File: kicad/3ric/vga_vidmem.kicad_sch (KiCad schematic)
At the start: 9 parts

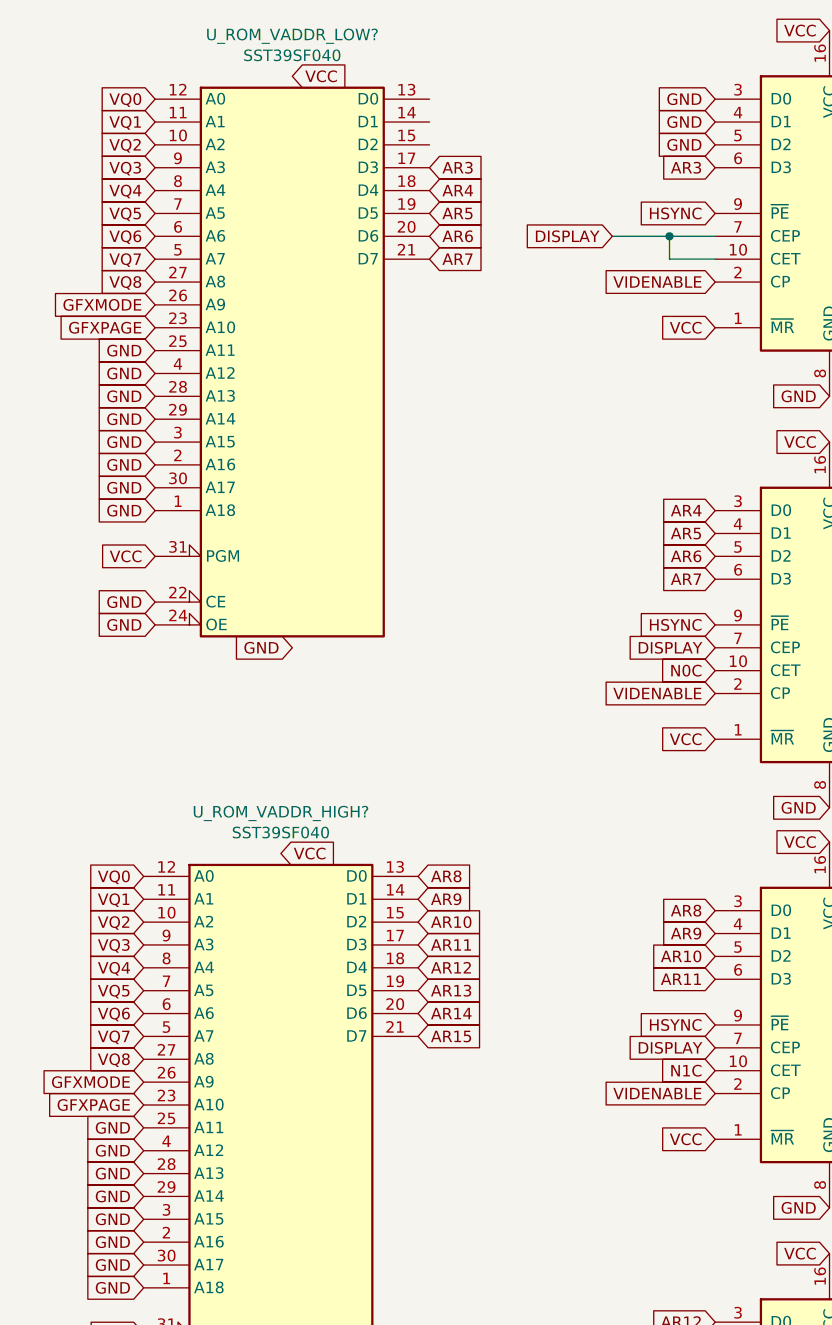
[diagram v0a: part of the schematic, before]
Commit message: updates to logisim project and schematics
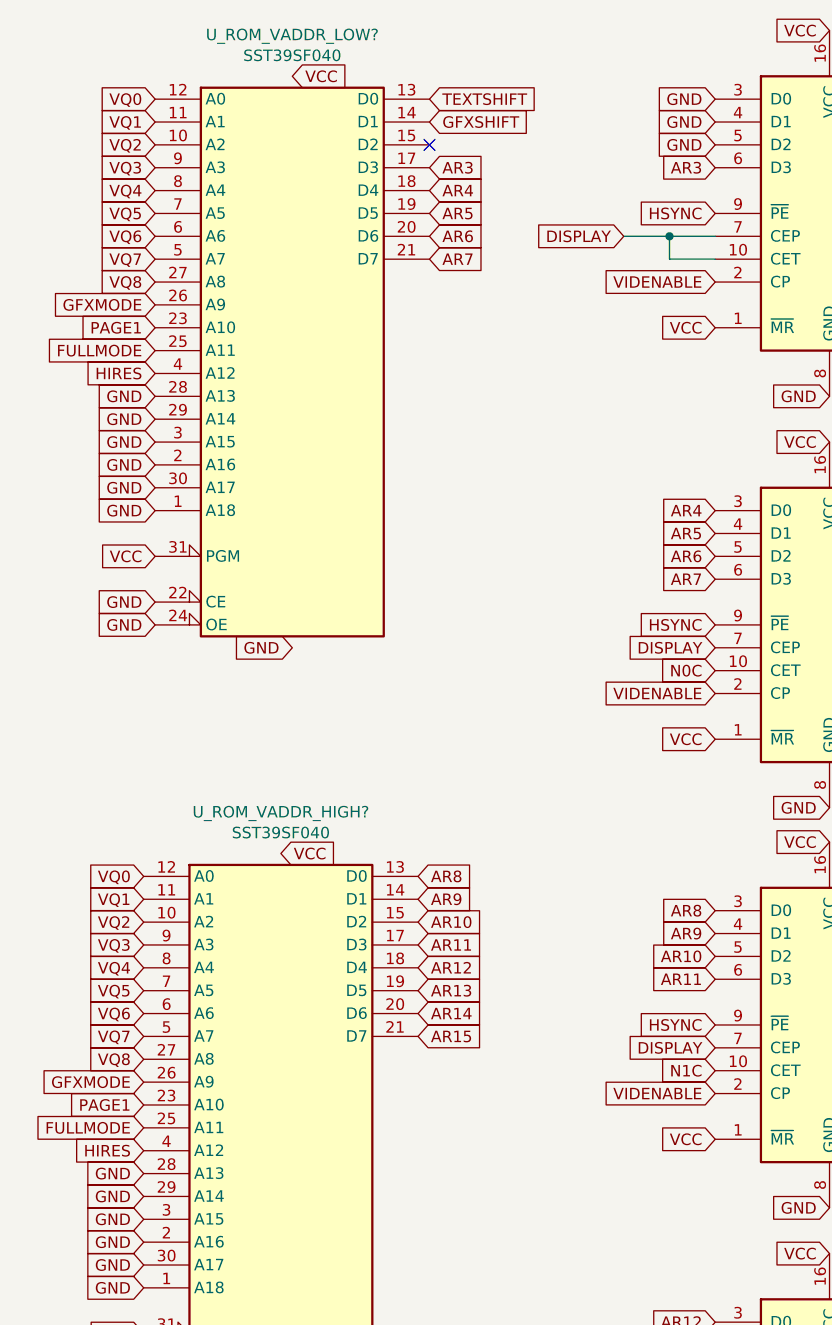
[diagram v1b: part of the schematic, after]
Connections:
- net GND: no longer U_ROM_VADDR_HIGH?.25 (A11), U_ROM_VADDR_HIGH?.4 (A12), U_ROM_VADDR_LOW?.25 (A11), U_ROM_VADDR_LOW?.4 (A12)
- net TEXTSHIFT: now reaches U_ROM_VADDR_LOW?.13 (D0)
- net GFXSHIFT: now reaches U_ROM_VADDR_LOW?.14 (D1)
- net GFXPAGE renamed PAGE1
- new net FULLMODE: U_ROM_VADDR_HIGH?.25 (A11), U_ROM_VADDR_LOW?.25 (A11)
- new net HIRES: U_ROM_VADDR_HIGH?.4 (A12), U_ROM_VADDR_LOW?.4 (A12)
- no-connect marks 1 -> 2
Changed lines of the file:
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@@
   )
   (no_connect (at 129.54 173.99))
+  (no_connect (at 72.39 30.48))
   (wire (pts (xy 143.51 76.2) (xy 143.51 63.5))
     (stroke (width 0) (type default) (color 0 0 0 0))
@@
     (stroke (width 0) (type default) (color 0 0 0 0))
   )
-  (wire (pts (xy 92.71 40.64) (xy 99.06 40.64))
+  (wire (pts (xy 93.98 40.64) (xy 99.06 40.64))
     (stroke (width 0) (type default) (color 0 0 0 0))
   )
@@
     )
   )
+  (global_label "HIRES" (shape input) (at 40.64 142.24 180) (fields_autoplaced)
+    (effects (font (size 1.27 1.27)) (justify right))
+    (property "Intersheet References" "${INTERSHEET_REFS}" (id 0) (at 32.6631 142.1606 0)
+      (effects (font (size 1.27 1.27)) (justify right) hide)
+    )
+  )
   (global_label "VQ1" (shape input) (at 41.91 27.94 180) (fields_autoplaced)
     (effects (font (size 1.27 1.27)) (justify right))
@@
     )
   )
+  (global_label "PAGE1" (shape input) (at 40.64 137.16 180) (fields_autoplaced)
+    (effects (font (size 1.27 1.27)) (justify right))
+    (property "Intersheet References" "${INTERSHEET_REFS}" (id 0) (at 32.2398 137.0806 0)
+      (effects (font (size 1.27 1.27)) (justify right) hide)
+    )
+  )
   (global_label "VD0" (shape input) (at 204.47 87.63 180) (fields_autoplaced)
     (effects (font (size 1.27 1.27)) (justify right))
@@
     )
   )
+  (global_label "TEXTSHIFT" (shape input) (at 72.39 25.4 0) (fields_autoplaced)
+    (effects (font (size 1.27 1.27)) (justify left))
+    (property "Intersheet References" "${INTERSHEET_REFS}" (id 0) (at 84.2979 25.3206 0)
+      (effects (font (size 1.27 1.27)) (justify left) hide)
+    )
+  )
   (global_label "VA3" (shape input) (at 177.8 55.88 0) (fields_autoplaced)
     (effects (font (size 1.27 1.27)) (justify left))
@@
     )
   )
-  (global_label "GFXPAGE" (shape input) (at 41.91 50.8 180) (fields_autoplaced)
-    (effects (font (size 1.27 1.27)) (justify right))
-    (property "Intersheet References" "${INTERSHEET_REFS}" (id 0) (at 31.1512 50.7206 0)
+  (global_label "PAGE1" (shape input) (at 41.91 50.8 180) (fields_autoplaced)
+    (effects (font (size 1.27 1.27)) (justify right))
+    (property "Intersheet References" "${INTERSHEET_REFS}" (id 0) (at 33.5098 50.7206 0)
       (effects (font (size 1.27 1.27)) (justify right) hide)
     )
@@
     )
   )
-  (global_label "GND" (shape input) (at 40.64 139.7 180) (fields_autoplaced)
-    (effects (font (size 1.27 1.27)) (justify right))
-    (property "Intersheet References" "${INTERSHEET_REFS}" (id 0) (at 34.3564 139.7794 0)
-      (effects (font (size 1.27 1.27)) (justify right) hide)
-    )
-  )
   (global_label "VQ2" (shape input) (at 41.91 30.48 180) (fields_autoplaced)
     (effects (font (size 1.27 1.27)) (justify right))
@@
     )
   )
+  (global_label "GFXSHIFT" (shape input) (at 72.39 27.94 0) (fields_autoplaced)
+    (effects (font (size 1.27 1.27)) (justify left))
+    (property "Intersheet References" "${INTERSHEET_REFS}" (id 0) (at 83.5721 27.8606 0)
+      (effects (font (size 1.27 1.27)) (justify left) hide)
+    )
+  )
   (global_label "VQ0" (shape input) (at 41.91 25.4 180) (fields_autoplaced)
     (effects (font (size 1.27 1.27)) (justify right))
@@
     )
   )
+  (global_label "GFXMODE" (shape input) (at 40.64 134.62 180) (fields_autoplaced)
+    (effects (font (size 1.27 1.27)) (justify right))
+    (property "Intersheet References" "${INTERSHEET_REFS}" (id 0) (at 29.4579 134.5406 0)
+      (effects (font (size 1.27 1.27)) (justify right) hide)
+    )
+  )
   (global_label "AR12" (shape input) (at 71.12 121.92 0) (fields_autoplaced)
     (effects (font (size 1.27 1.27)) (justify left))
@@
     )
   )
-  (global_label "GFXMODE" (shape input) (at 40.64 134.62 180) (fields_autoplaced)
-    (effects (font (size 1.27 1.27)) (justify right))
-    (property "Intersheet References" "${INTERSHEET_REFS}" (id 0) (at 29.4579 134.5406 0)
-      (effects (font (size 1.27 1.27)) (justify right) hide)
-    )
-  )
   (global_label "VCC" (shape input) (at 217.17 80.01 90) (fields_autoplaced)
     (effects (font (size 1.27 1.27)) (justify left))
@@
     )
   )
-  (global_label "GND" (shape input) (at 40.64 142.24 180) (fields_autoplaced)
-    (effects (font (size 1.27 1.27)) (justify right))
-    (property "Intersheet References" "${INTERSHEET_REFS}" (id 0) (at 34.3564 142.1606 0)
-      (effects (font (size 1.27 1.27)) (justify right) hide)
-    )
-  )
   (global_label "VMLATCH" (shape input) (at 204.47 110.49 180) (fields_autoplaced)
     (effects (font (size 1.27 1.27)) (justify right))
@@
     )
   )
-  (global_label "GFXPAGE" (shape input) (at 40.64 137.16 180) (fields_autoplaced)
-    (effects (font (size 1.27 1.27)) (justify right))
-    (property "Intersheet References" "${INTERSHEET_REFS}" (id 0) (at 29.8812 137.0806 0)
-      (effects (font (size 1.27 1.27)) (justify right) hide)
-    )
-  )
-  (global_label "GND" (shape input) (at 41.91 55.88 180) (fields_autoplaced)
-    (effects (font (size 1.27 1.27)) (justify right))
-    (property "Intersheet References" "${INTERSHEET_REFS}" (id 0) (at 35.6264 55.9594 0)
-      (effects (font (size 1.27 1.27)) (justify right) hide)
-    )
-  )
   (global_label "VA11" (shape input) (at 177.8 135.89 0) (fields_autoplaced)
     (effects (font (size 1.27 1.27)) (justify left))
@@
     )
   )
-  (global_label "GND" (shape input) (at 41.91 53.34 180) (fields_autoplaced)
-    (effects (font (size 1.27 1.27)) (justify right))
-    (property "Intersheet References" "${INTERSHEET_REFS}" (id 0) (at 35.6264 53.4194 0)
+  (global_label "FULLMODE" (shape input) (at 41.91 53.34 180) (fields_autoplaced)
+    (effects (font (size 1.27 1.27)) (justify right))
+    (property "Intersheet References" "${INTERSHEET_REFS}" (id 0) (at 29.8207 53.2606 0)
       (effects (font (size 1.27 1.27)) (justify right) hide)
     )
@@
     )
   )
-  (global_label "DISPLAY" (shape input) (at 92.71 40.64 180) (fields_autoplaced)
-    (effects (font (size 1.27 1.27)) (justify right))
-    (property "Intersheet References" "${INTERSHEET_REFS}" (id 0) (at 82.7374 40.5606 0)
+  (global_label "DISPLAY" (shape input) (at 93.98 40.64 180) (fields_autoplaced)
+    (effects (font (size 1.27 1.27)) (justify right))
+    (property "Intersheet References" "${INTERSHEET_REFS}" (id 0) (at 84.0074 40.5606 0)
       (effects (font (size 1.27 1.27)) (justify right) hide)
     )
@@
     )
   )
+  (global_label "HIRES" (shape input) (at 41.91 55.88 180) (fields_autoplaced)
+    (effects (font (size 1.27 1.27)) (justify right))
+    (property "Intersheet References" "${INTERSHEET_REFS}" (id 0) (at 33.9331 55.8006 0)
+      (effects (font (size 1.27 1.27)) (justify right) hide)
+    )
+  )
   (global_label "VCC" (shape input) (at 165.1 40.64 90) (fields_autoplaced)
     (effects (font (size 1.27 1.27)) (justify left))
@@
     )
   )
+  (global_label "FULLMODE" (shape input) (at 40.64 139.7 180) (fields_autoplaced)
+    (effects (font (size 1.27 1.27)) (justify right))
+    (property "Intersheet References" "${INTERSHEET_REFS}" (id 0) (at 28.5507 139.6206 0)
+      (effects (font (size 1.27 1.27)) (justify right) hide)
+    )
+  )

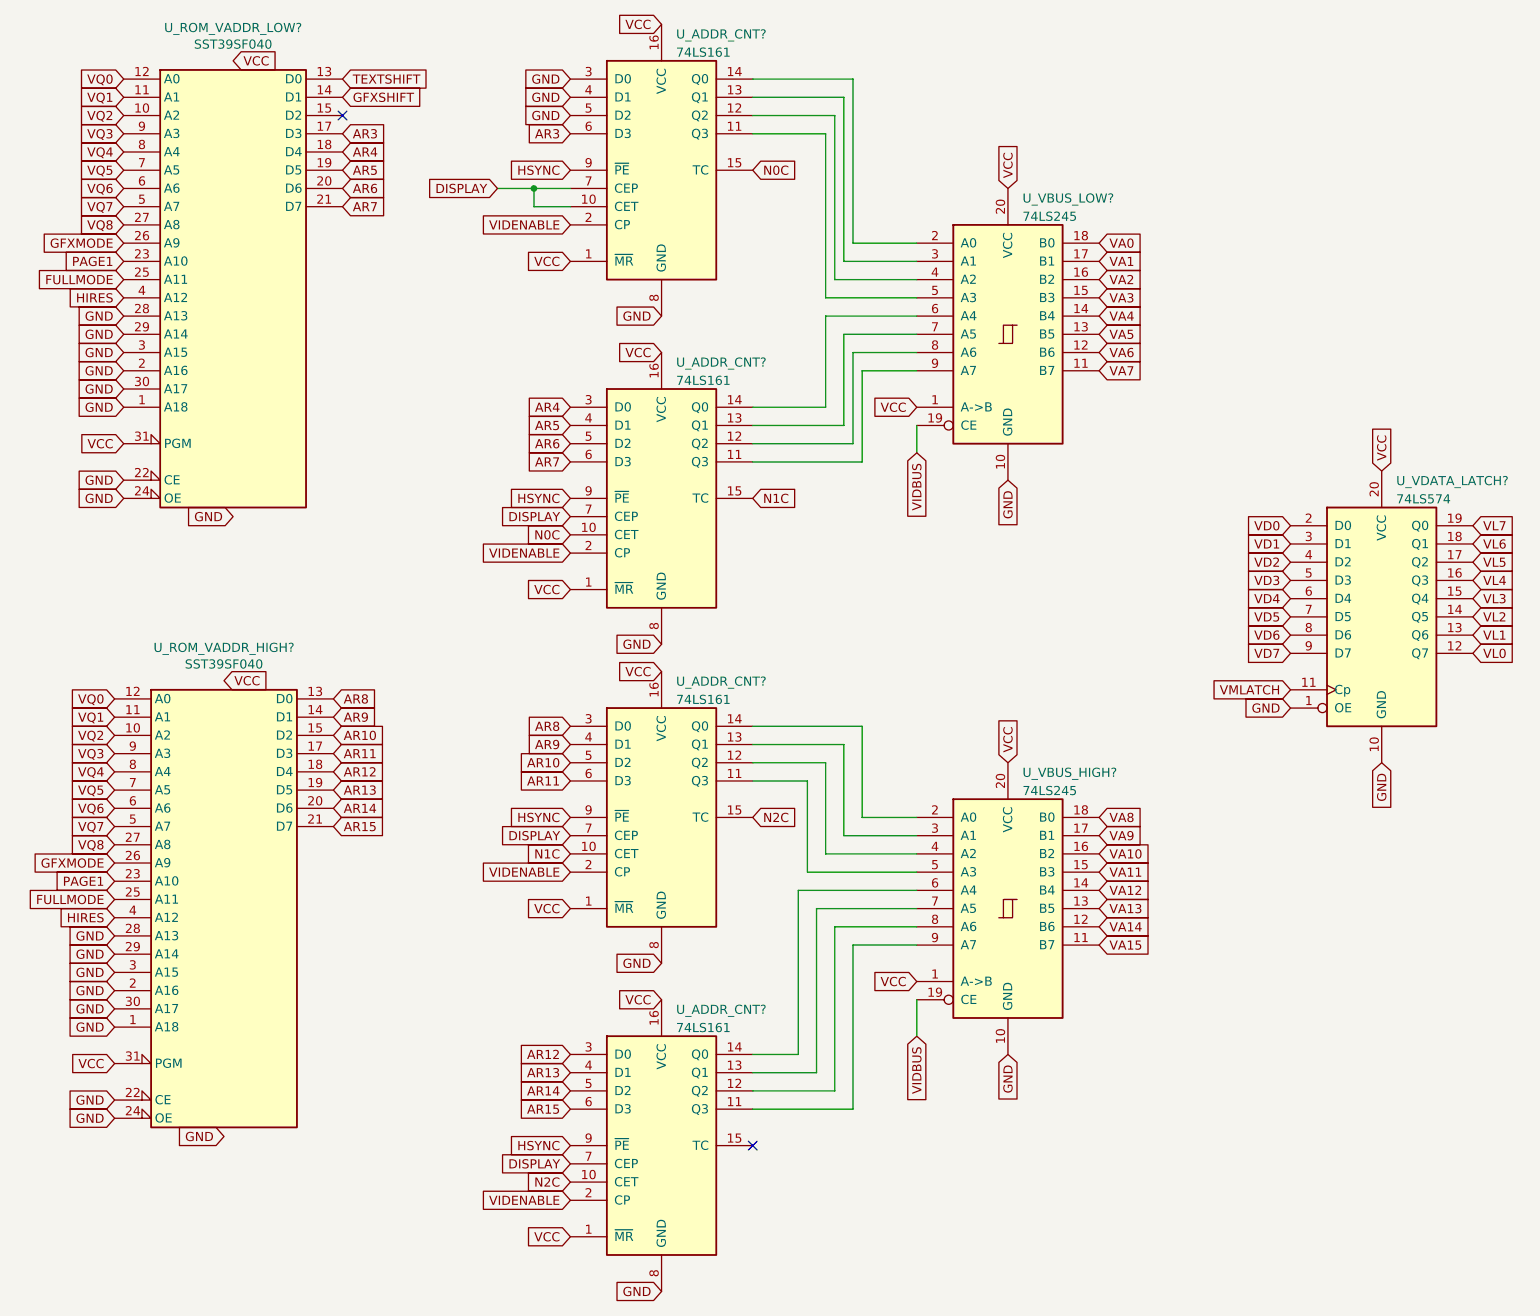
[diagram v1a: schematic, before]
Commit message: push schematic updates
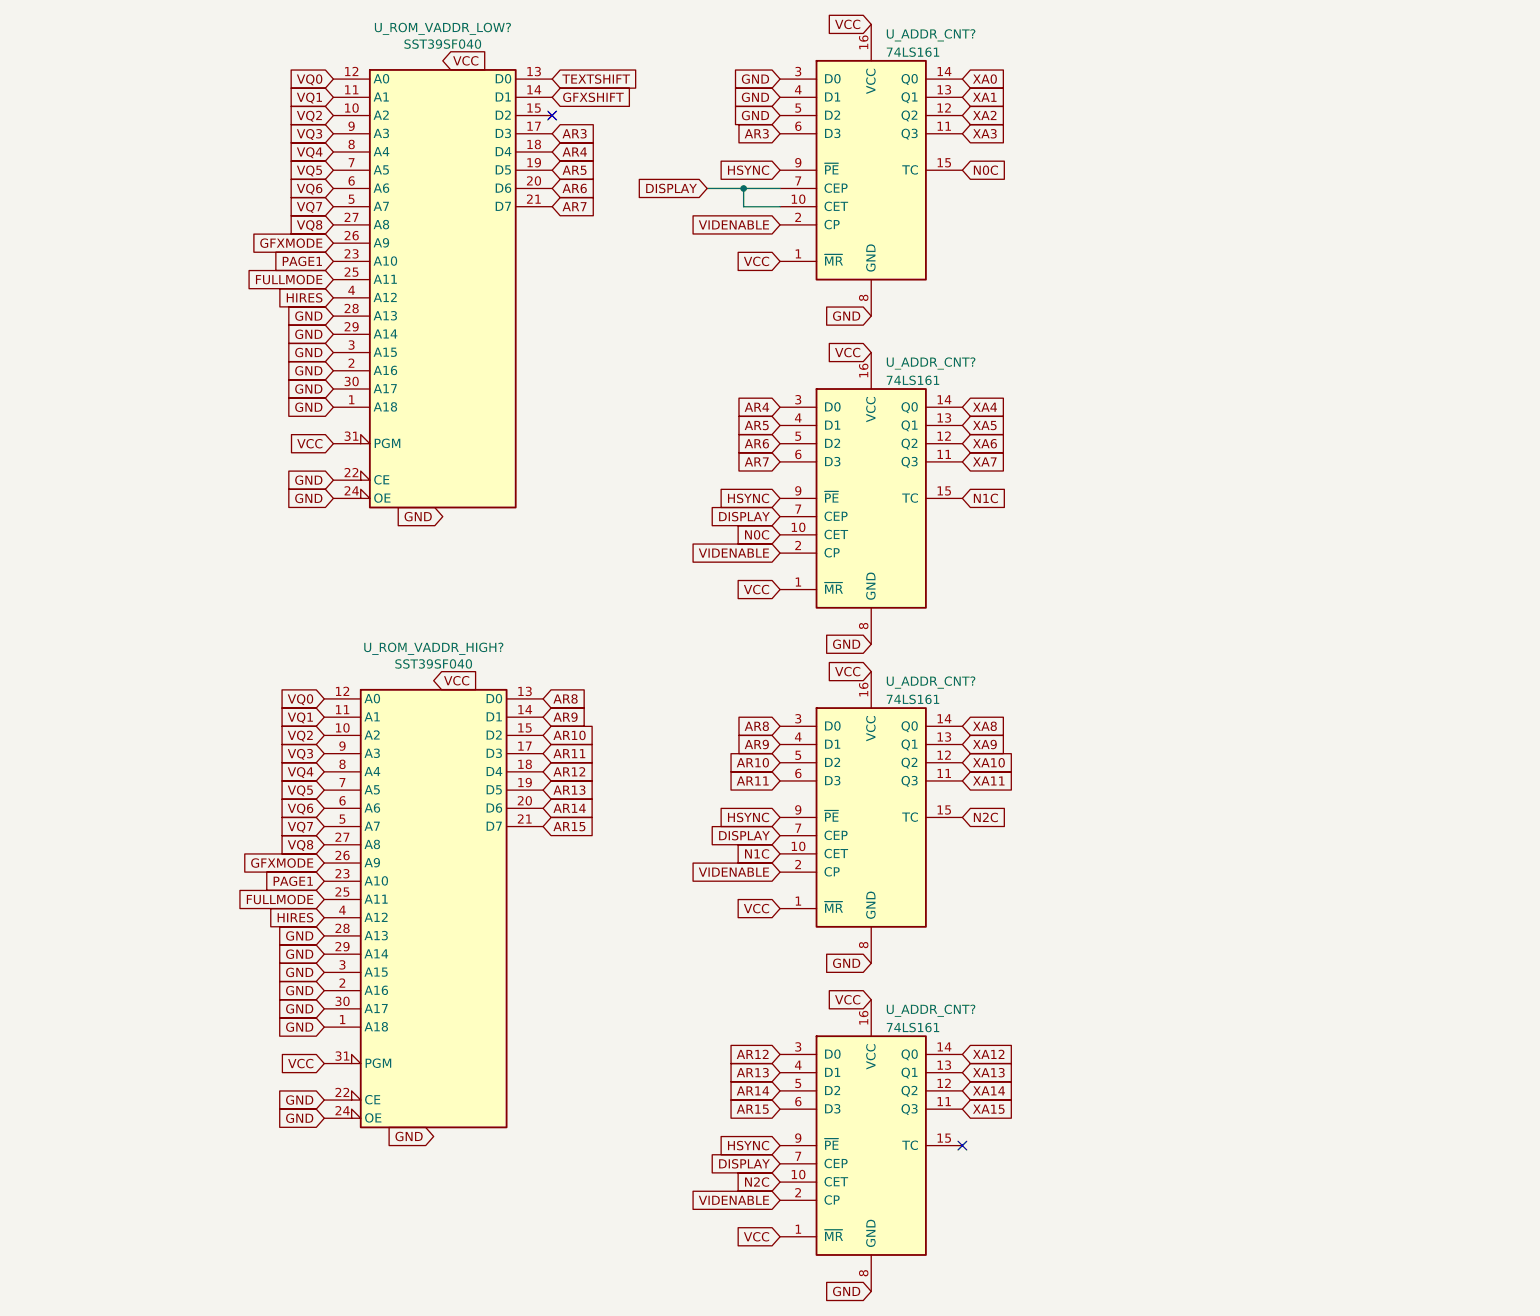
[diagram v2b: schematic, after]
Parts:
- removed U_VBUS_HIGH?, U_VBUS_LOW?: 74LS245, Package_DIP:DIP-20_W7.62mm_Socket, symbol 74xx:74LS245
- removed U_VDATA_LATCH?: 74LS574, Package_DIP:DIP-20_W7.62mm_Socket, symbol 74xx:74LS574
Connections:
- net XA8: now reaches U_ADDR_CNT?.14 (Q0)
- net XA9: now reaches U_ADDR_CNT?.13 (Q1)
- net XA10: now reaches U_ADDR_CNT?.12 (Q2)
- net XA11: now reaches U_ADDR_CNT?.11 (Q3)
- net XA12: now reaches U_ADDR_CNT?.14 (Q0)
- net XA13: now reaches U_ADDR_CNT?.13 (Q1)
- net XA14: now reaches U_ADDR_CNT?.12 (Q2)
- net XA15: now reaches U_ADDR_CNT?.11 (Q3)
- net XA0: now reaches U_ADDR_CNT?.14 (Q0)
- net XA1: now reaches U_ADDR_CNT?.13 (Q1)
- net XA2: now reaches U_ADDR_CNT?.12 (Q2)
- net XA3: now reaches U_ADDR_CNT?.11 (Q3)
- net XA4: now reaches U_ADDR_CNT?.14 (Q0)
- net XA5: now reaches U_ADDR_CNT?.13 (Q1)
- net XA6: now reaches U_ADDR_CNT?.12 (Q2)
- net XA7: now reaches U_ADDR_CNT?.11 (Q3)
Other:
- moved on the sheet: U_ADDR_CNT?, U_ROM_VADDR_HIGH?, U_ROM_VADDR_LOW?
